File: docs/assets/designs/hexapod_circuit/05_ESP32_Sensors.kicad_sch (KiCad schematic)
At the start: 29 parts, among them U3 ESP32, U4 SN65HVD230

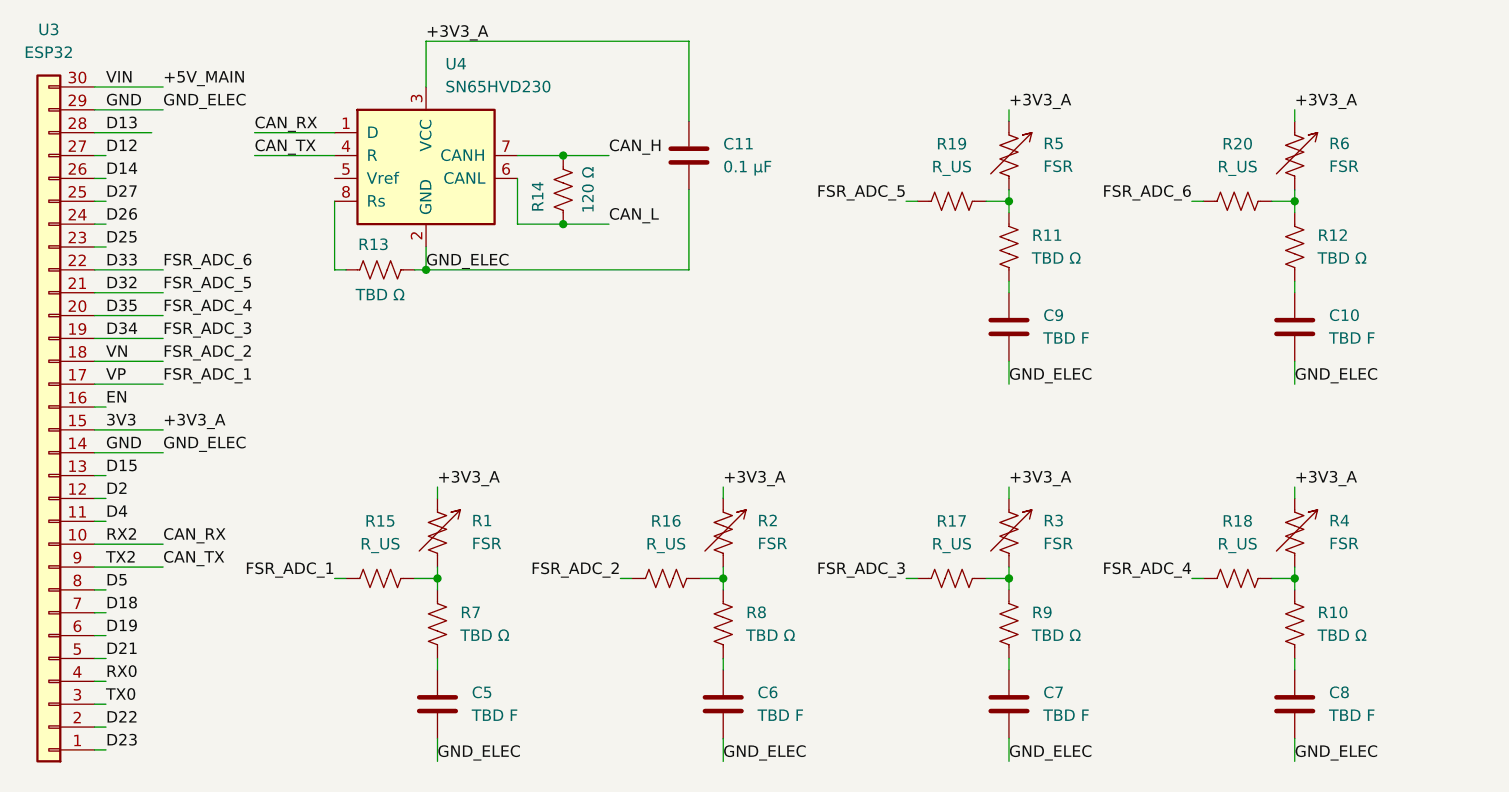
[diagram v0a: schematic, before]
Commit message: Add files via upload
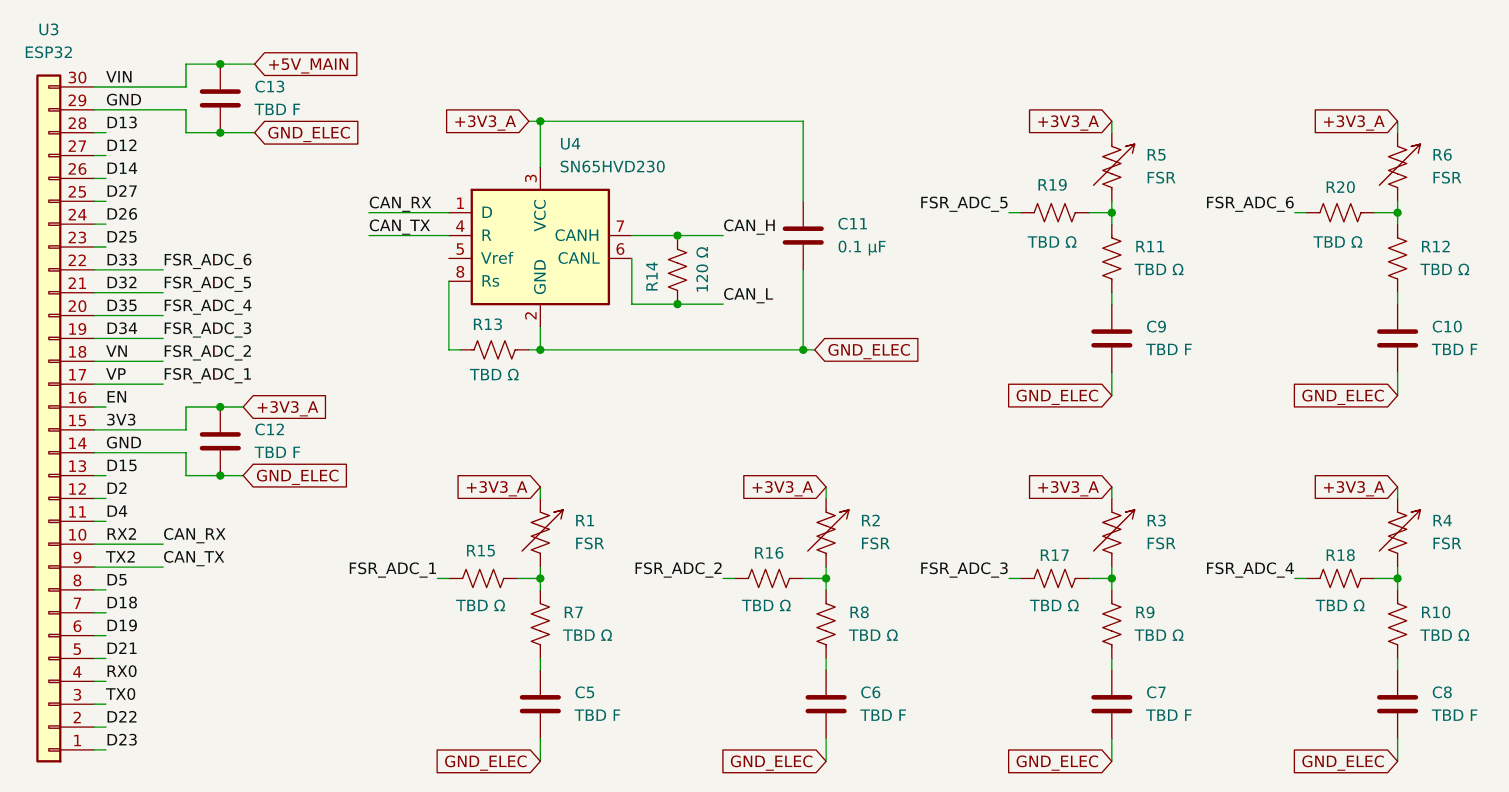
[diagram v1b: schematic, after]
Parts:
- added C12, C13: TBD F, symbol Device:C
- R15, R16, R17, R18, R19, R20: value R_US -> TBD Ω
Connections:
- net +3V3_A: now also C12.1
- net +5V_MAIN: now also C13.1
- net GND renamed GND_ELEC
- net GND_ELEC: now also C12.2, C13.2
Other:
- moved on the sheet: C10, C11, C5, C6, C7, C8, C9, R1, R10, R11, R12, R13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
